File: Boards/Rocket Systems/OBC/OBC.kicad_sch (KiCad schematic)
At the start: 68 parts, among them IC1 NSVT30010MXV6T1G, IC2 BC846BLT1G, J1 1718560006, J2 5023520200, J3 MEM2061-01-188-00-A_REVA, J4 SMARA_CONNECTOR, U1 SX1280IMLTRT, U2 STLM20DD9F, U3 NRF21540-QDAA-R, U4 THVD2410VDRCR, U5 VLMKG3400-GS08

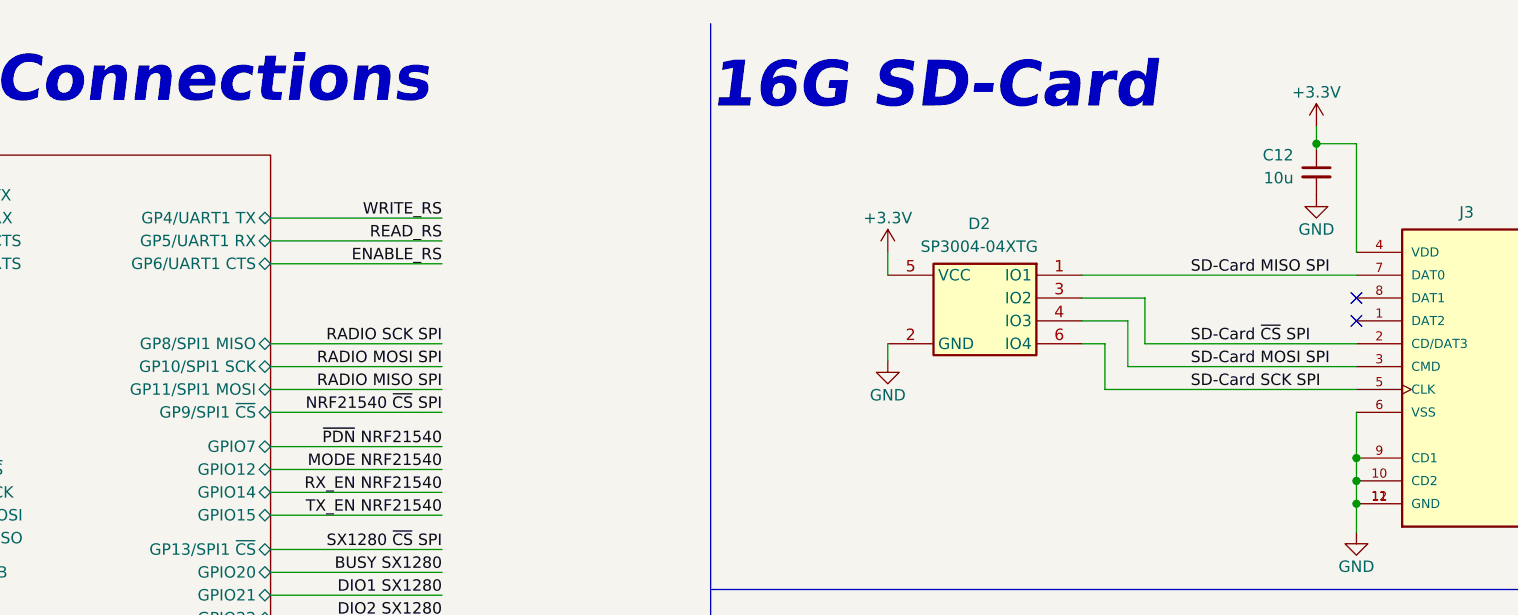
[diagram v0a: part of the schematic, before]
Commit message: New OBC PCB project
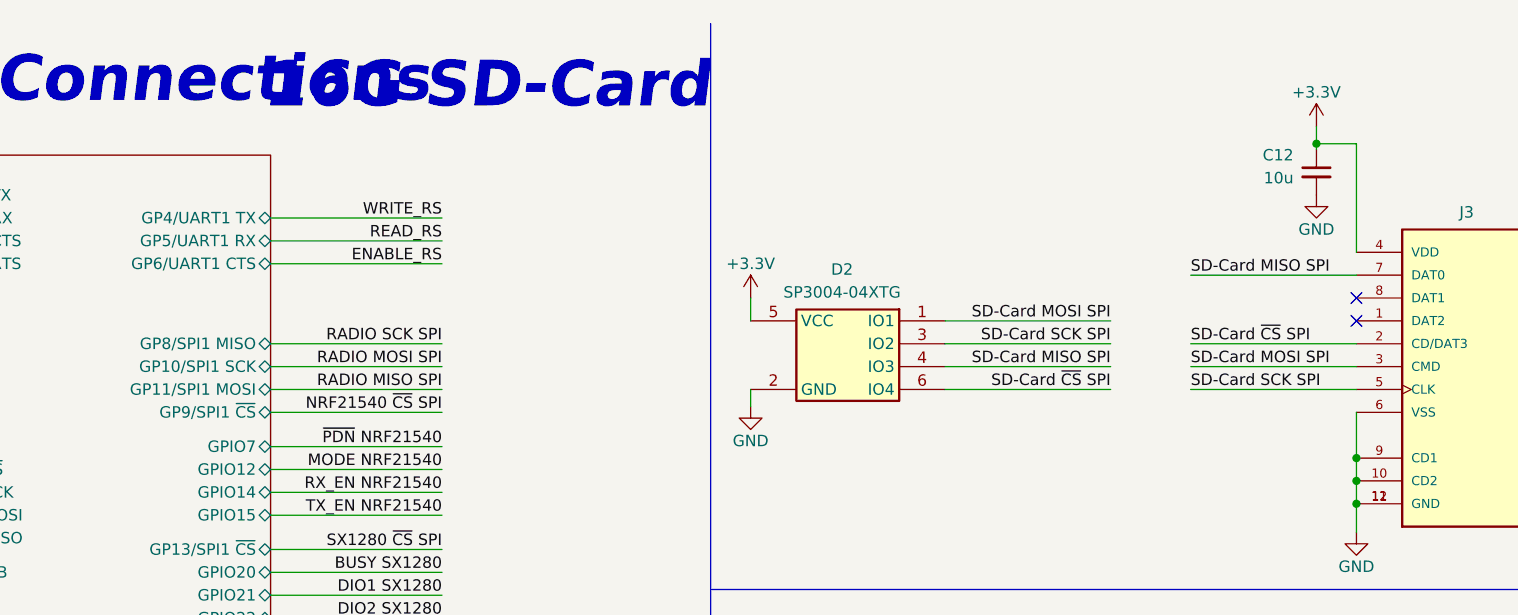
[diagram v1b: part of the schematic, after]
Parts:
- R13, R14, R4, R5, R6, R7: footprint Resistor-0402:RES_0402 -> Resistor-0603:RES_0603
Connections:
- net SD-Card  ~{CS} SPI: now also D2.6 (IO4); no longer D2.3 (IO2)
- net SD-Card MISO SPI: now also D2.4 (IO3); no longer D2.1 (IO1)
- net SD-Card MOSI SPI: now also D2.1 (IO1); no longer D2.4 (IO3)
- net SD-Card SCK SPI: now also D2.3 (IO2); no longer D2.6 (IO4)
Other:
- moved on the sheet: D2

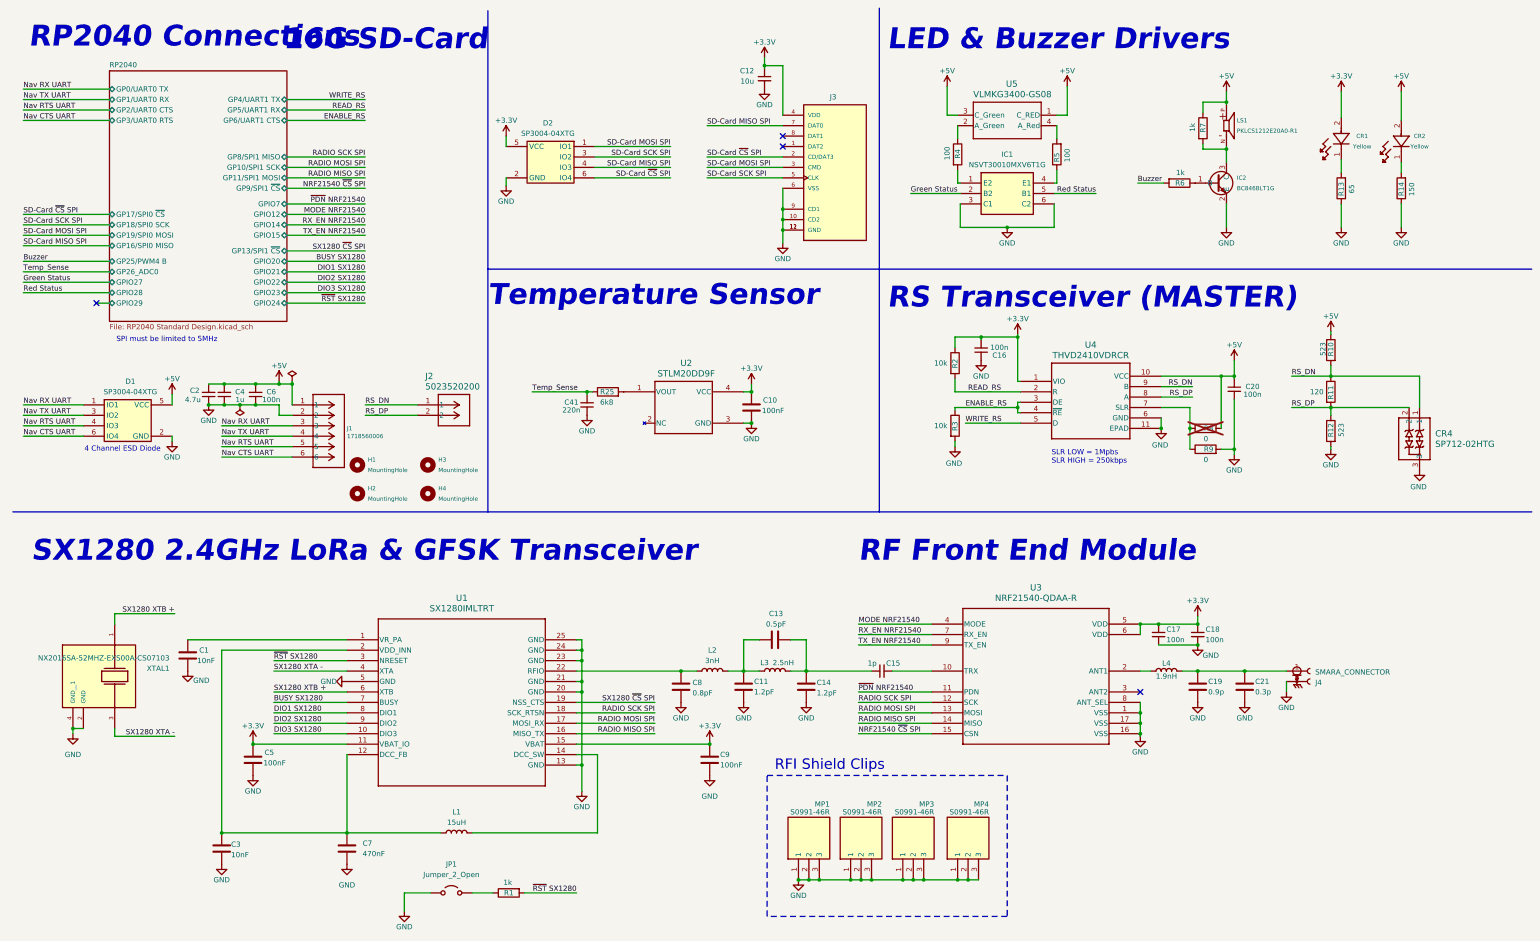
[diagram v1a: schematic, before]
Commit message: Nav & OBC update
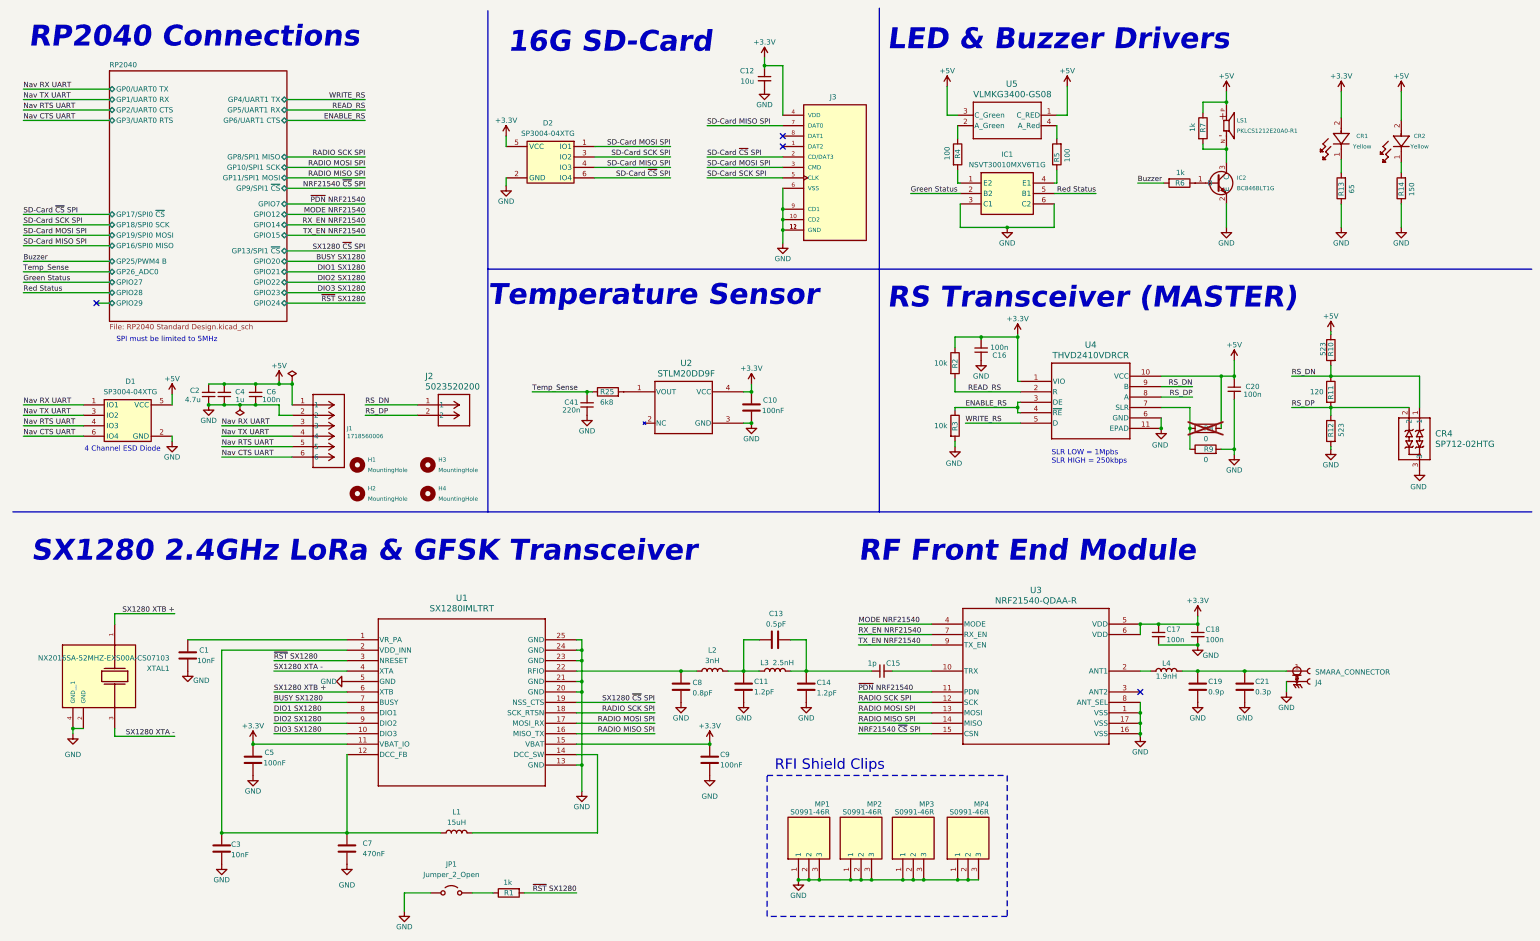
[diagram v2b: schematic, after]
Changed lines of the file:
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@@
 	(text "16G SD-Card"
 		(exclude_from_sim no)
-		(at 127.635 19.685 0)
+		(at 182.245 20.32 0)
 		(effects
 			(font
@@
 		(fields_autoplaced yes)
 		(property "Reference" "U3"
-			(at 260.985 153.035 0)
+			(at 260.985 153.67 0)
 			(effects
 				(font
@@
 		)
 		(property "Value" "NRF21540-QDAA-R"
-			(at 260.985 155.575 0)
+			(at 260.985 156.21 0)
 			(effects
 				(font
